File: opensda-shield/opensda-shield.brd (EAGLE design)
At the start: 21.6 x 53.3 mm, 17 parts, among them IC1 74LVC125, IC2 74LVC125, J1 61302011121, J2 61302011121, J3 61300211121, J4 CORTEX_DEBUG_PTH, J5 61301511121

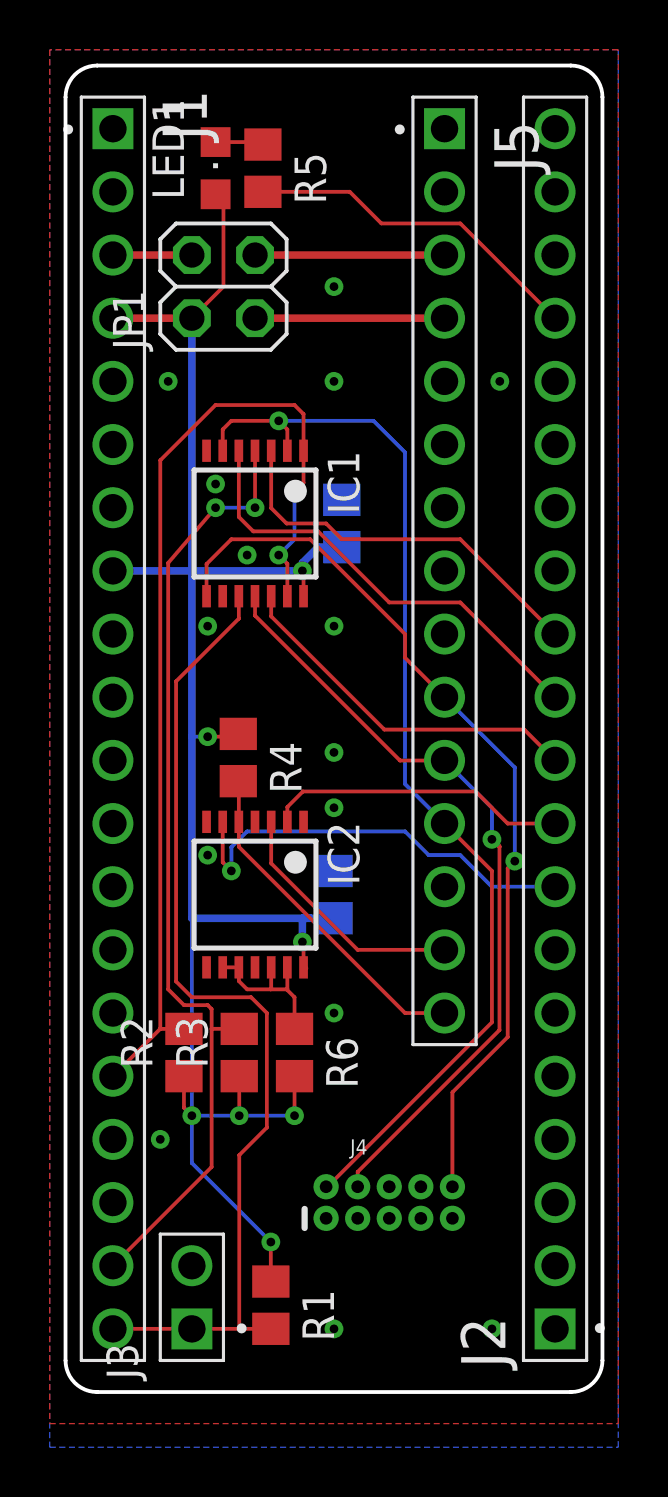
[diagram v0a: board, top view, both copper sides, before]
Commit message: Zmeny z e-mailu
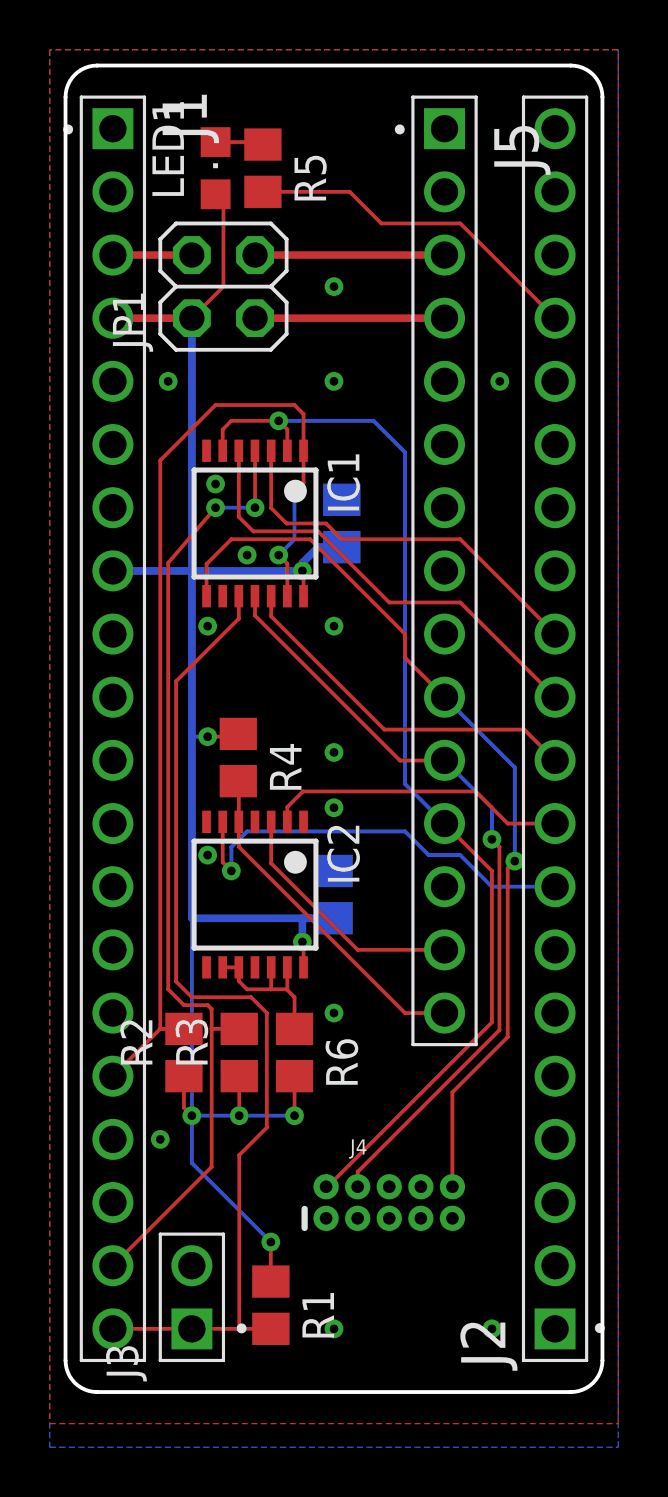
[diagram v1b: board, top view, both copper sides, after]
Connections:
- net N$1 renamed 3V3_OUT
- net N$3 renamed USB5V_OUT
- net PTA4 renamed !SDA_SWD_EN_PTA4
- net PTB0 renamed !SDA_SWD_OE_PTB0
- net PTB1 renamed !SDA_RST_TGTMCU_PTB1
- net PTC3 renamed UART0_TX_TGTMCU_PTC3
- net PTC4 renamed UART0_RX_TGTMCU_PTC4
- net PTC5 renamed SDA_SPI0_SCK_PTC5
- net PTC6 renamed SDA_SPI0_SOUT_PTC6
- net PTC7 renamed SDA_SPI0_SIN_PTC7
- net PTD4 renamed !SDA_LED_PTD4
- net RST_TGT renamed !RST_TGT
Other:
- board text removed: "PTB1"
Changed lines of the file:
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@@
 <layer number="23" name="tOrigins" color="15" fill="1" visible="yes" active="yes"/>
 <layer number="24" name="bOrigins" color="15" fill="1" visible="yes" active="yes"/>
-<layer number="25" name="tNames" color="7" fill="1" visible="yes" active="yes"/>
-<layer number="26" name="bNames" color="7" fill="1" visible="yes" active="yes"/>
+<layer number="25" name="tNames" color="7" fill="1" visible="no" active="yes"/>
+<layer number="26" name="bNames" color="7" fill="1" visible="no" active="yes"/>
 <layer number="27" name="tValues" color="7" fill="1" visible="no" active="yes"/>
 <layer number="28" name="bValues" color="7" fill="1" visible="no" active="yes"/>
@@
 <text x="13.97" y="15.24" size="1.016" layer="111" ratio="15" align="center-right">TX</text>
 <text x="7.3025" y="51.1175" size="1.016" layer="111" ratio="15" rot="R180" align="top-center">PTD4</text>
-<text x="9.525" y="2.54" size="1.016" layer="111" ratio="15" rot="R180" align="center-right">PTB1</text>
 <circle x="10.795" y="37.7825" radius="0.254" width="0.1524" layer="111"/>
 <circle x="10.795" y="22.86" radius="0.254" width="0.1524" layer="111"/>
@@
 <contactref element="C2" pad="1"/>
 <wire x1="1.905" y1="43.18" x2="5.08" y2="43.18" width="0.3048" layer="1"/>
-<wire x1="9.60755" y1="17.03995" x2="9.57" y2="17.0775" width="0.3048" layer="1"/>
 <wire x1="5.08" y1="43.18" x2="6.35" y2="44.45" width="0.1524" layer="1"/>
 <wire x1="6.35" y1="47.845" x2="6.0325" y2="48.1625" width="0.1524" layer="1"/>
@@
 <contactref element="J1" pad="15"/>
 </signal>
-<signal name="PTA4">
+<signal name="!SDA_SWD_EN_PTA4">
 <contactref element="J1" pad="16"/>
 <contactref element="R2" pad="2"/>
@@
 <contactref element="J1" pad="18"/>
 </signal>
-<signal name="PTB0">
+<signal name="!SDA_SWD_OE_PTB0">
 <contactref element="J1" pad="19"/>
 <contactref element="R3" pad="2"/>
 <contactref element="IC1" pad="4"/>
-<wire x1="7.62" y1="37.85" x2="7.62" y2="35.56" width="0.1524" layer="1"/>
-<wire x1="7.62" y1="35.56" x2="7.619996875" y2="35.559996875" width="0.1524" layer="1"/>
 <via x="6.0325" y="35.56" extent="1-16" drill="0.35"/>
-<wire x1="7.62" y1="35.56" x2="6.0325" y2="35.56" width="0.1524" layer="16"/>
-<via x="7.62" y="35.56" extent="1-16" drill="0.35"/>
+<wire x1="6.0325" y1="35.56" x2="7.62" y2="35.56" width="0.1524" layer="16"/>
 <wire x1="4.1275" y1="33.3375" x2="6.0325" y2="35.56" width="0.1524" layer="1"/>
 <wire x1="5.87375" y1="9.04875" x2="1.905" y2="5.08" width="0.1524" layer="1"/>
@@
 <wire x1="5.87375" y1="15.39875" x2="5.715" y2="15.5575" width="0.1524" layer="1"/>
 <wire x1="5.715" y1="15.5575" x2="4.7625" y2="15.5575" width="0.1524" layer="1"/>
-</signal>
-<signal name="PTB1">
+<via x="7.62" y="35.56" extent="1-16" drill="0.35"/>
+<wire x1="7.62" y1="35.56" x2="7.62" y2="37.85" width="0.1524" layer="1"/>
+</signal>
+<signal name="!SDA_RST_TGTMCU_PTB1">
 <contactref element="J1" pad="20"/>
 <contactref element="R1" pad="2"/>
@@
 <contactref element="J2" pad="7"/>
 </signal>
-<signal name="PTC3">
+<signal name="UART0_TX_TGTMCU_PTC3">
 <contactref element="J2" pad="8"/>
 <contactref element="IC2" pad="6"/>
@@
 <wire x1="6.6675" y1="20.955" x2="6.6675" y2="21.9075" width="0.1524" layer="16"/>
 </signal>
-<signal name="PTC4">
+<signal name="UART0_RX_TGTMCU_PTC4">
 <contactref element="J2" pad="9"/>
 <contactref element="IC2" pad="2"/>
@@
 <wire x1="9.54405" y1="24.14905" x2="16.49095" y2="24.14905" width="0.1524" layer="1"/>
 </signal>
-<signal name="PTC5">
+<signal name="SDA_SPI0_SCK_PTC5">
 <contactref element="J2" pad="10"/>
 <wire x1="18.44675" y1="26.63825" x2="19.685" y2="25.4" width="0.1524" layer="1"/>
@@
 <wire x1="8.27" y1="31.1889" x2="12.82065" y2="26.63825" width="0.1524" layer="1"/>
 </signal>
-<signal name="PTC6">
+<signal name="SDA_SPI0_SOUT_PTC6">
 <contactref element="J2" pad="11"/>
 <contactref element="IC1" pad="5"/>
@@
 <wire x1="15.875" y1="31.75" x2="13.0175" y2="31.75" width="0.1524" layer="1"/>
 </signal>
-<signal name="PTC7">
+<signal name="SDA_SPI0_SIN_PTC7">
 <contactref element="J2" pad="12"/>
 <contactref element="IC1" pad="3"/>
@@
 <contactref element="J2" pad="16"/>
 </signal>
-<signal name="PTD4">
+<signal name="!SDA_LED_PTD4">
 <contactref element="J2" pad="17"/>
 <contactref element="R5" pad="2"/>
@@
 <wire x1="15.23365" y1="25.39365" x2="13.4493" y2="25.39365" width="0.1524" layer="1"/>
 <wire x1="7.62" y1="31.22295" x2="13.4493" y2="25.39365" width="0.1524" layer="1"/>
-<wire x1="17.4498" y1="21.971" x2="17.4498" y2="21.9202" width="0.1524" layer="1"/>
 <wire x1="17.4498" y1="21.9202" x2="17.4498" y2="14.5542" width="0.1524" layer="1"/>
 <wire x1="11.7475" y1="8.255" x2="11.7475" y2="8.8519" width="0.1524" layer="1"/>
@@
 <wire x1="17.145" y1="22.225" x2="17.4498" y2="21.9202" width="0.1524" layer="1"/>
 </signal>
-<signal name="RST_TGT">
+<signal name="!RST_TGT">
 <contactref element="J5" pad="10"/>
 <contactref element="J4" pad="10"/>
@@
 <contactref element="IC2" pad="12"/>
 <wire x1="6.32" y1="17.0775" x2="6.97" y2="17.0775" width="0.1524" layer="1"/>
-<wire x1="9.2075" y1="14.6025" x2="9.17195" y2="14.6025" width="0.1524" layer="1"/>
-<wire x1="9.2075" y1="14.73205" x2="9.2075" y2="14.6025" width="0.1524" layer="1"/>
+<wire x1="9.2075" y1="14.73205" x2="9.2075" y2="14.605" width="0.1524" layer="1"/>
 <wire x1="8.255" y1="16.1925" x2="8.89" y2="16.1925" width="0.1524" layer="1"/>
-<wire x1="8.89" y1="16.1925" x2="8.92" y2="16.1925" width="0.1524" layer="1"/>
 <wire x1="8.92" y1="17.0775" x2="8.92" y2="16.2225" width="0.1524" layer="1"/>
 <wire x1="8.92" y1="16.2225" x2="8.89" y2="16.1925" width="0.1524" layer="1"/>
@@
 <wire x1="7.3025" y1="16.1925" x2="8.255" y2="16.1925" width="0.1524" layer="1"/>
 <wire x1="9.2075" y1="15.875" x2="8.89" y2="16.1925" width="0.1524" layer="1"/>
-<wire x1="9.2075" y1="14.6025" x2="9.2075" y2="15.875" width="0.1524" layer="1"/>
-</signal>
-<signal name="N$1">
+<wire x1="9.2075" y1="14.73205" x2="9.2075" y2="15.875" width="0.1524" layer="1"/>
+<wire x1="9.2075" y1="14.6025" x2="9.2075" y2="14.605" width="0.1524" layer="1"/>
+</signal>
+<signal name="3V3_OUT">
 <contactref element="J5" pad="3"/>
 <contactref element="JP1" pad="3"/>
 <wire x1="7.62" y1="45.72" x2="15.24" y2="45.72" width="0.3048" layer="1"/>
 </signal>
-<signal name="N$3">
+<signal name="USB5V_OUT">
 <contactref element="J5" pad="4"/>
 <contactref element="JP1" pad="1"/>
